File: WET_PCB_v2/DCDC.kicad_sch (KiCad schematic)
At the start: 8 parts, among them Q5 Q_NMOS_GDS, Q6 Q_NMOS_GDS

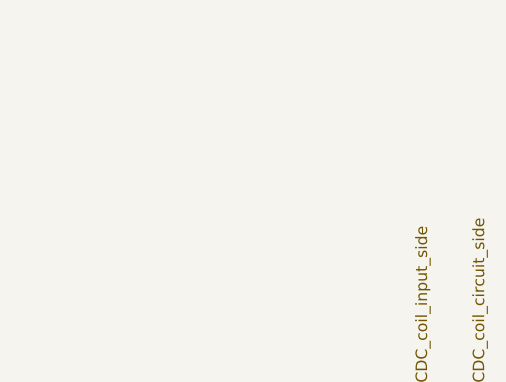
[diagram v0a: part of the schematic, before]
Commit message: finished and added some drawings
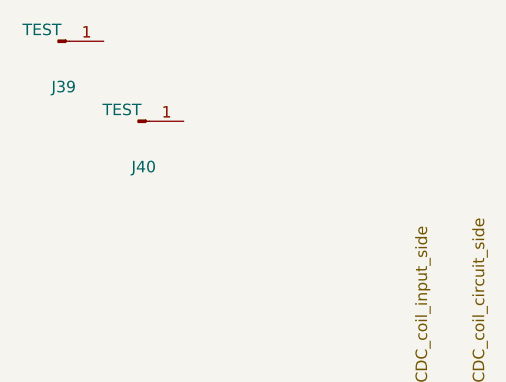
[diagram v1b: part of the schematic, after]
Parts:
- added J39, J40: TEST, Connector_PinSocket_2.54mm:PinSocket_1x01_P2.54mm_Vertical, symbol Connector:Conn_01x01_Pin
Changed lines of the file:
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@@
+	)
+	(symbol
+		(lib_id "Connector:Conn_01x01_Pin")
+		(at 12.926 11.1816 0)
+		(unit 1)
+		(body_style 1)
+		(exclude_from_sim no)
+		(in_bom yes)
+		(on_board yes)
+		(in_pos_files yes)
+		(dnp no)
+		(property "Reference" "J40"
+			(at 13.561 16.2616 0)
+			(show_name no)
+			(do_not_autoplace no)
+			(effects
+				(font
+					(size 1.27 1.27)
+				)
+			)
+		)
+		(property "Value" "TEST"
+			(at 11.148 9.9116 0)
+			(show_name no)
+			(do_not_autoplace no)
+			(effects
+				(font
+					(size 1.27 1.27)
+				)
+			)
+		)
+		(property "Footprint" "Connector_PinSocket_2.54mm:PinSocket_1x01_P2.54mm_Vertical"
+			(at 12.926 11.1816 0)
+			(hide yes)
+			(show_name no)
+			(do_not_autoplace no)
+			(effects
+				(font
+					(size 1.27 1.27)
+				)
+			)
+		)
+		(property "Datasheet" ""
+			(at 12.926 11.1816 0)
+			(hide yes)
+			(show_name no)
+			(do_not_autoplace no)
+			(effects
+				(font
+					(size 1.27 1.27)
+				)
+			)
+		)
+		(property "Description" "Generic connector, single row, 01x01, script generated"
+			(at 12.926 11.1816 0)
+			(hide yes)
+			(show_name no)
+			(do_not_autoplace no)
+			(effects
+				(font
+					(size 1.27 1.27)
+				)
+			)
+		)
+		(pin "1"
+		)
+		(instances
+			(project "WET_PCB_v2"
+				(path "/13451c35-1666-47d9-9525-8d8125ba1cf3/04007180-46fe-4cf0-9e6f-a7d321798318"
+					(reference "J40")
+					(unit 1)
+				)
+			)
+		)
+	)
+	(symbol
+		(lib_id "Connector:Conn_01x01_Pin")
+		(at 4.036 2.2916 0)
+		(unit 1)
+		(body_style 1)
+		(exclude_from_sim no)
+		(in_bom yes)
+		(on_board yes)
+		(in_pos_files yes)
+		(dnp no)
+		(property "Reference" "J39"
+			(at 4.671 7.3716 0)
+			(show_name no)
+			(do_not_autoplace no)
+			(effects
+				(font
+					(size 1.27 1.27)
+				)
+			)
+		)
+		(property "Value" "TEST"
+			(at 2.258 1.0216 0)
+			(show_name no)
+			(do_not_autoplace no)
+			(effects
+				(font
+					(size 1.27 1.27)
+				)
+			)
+		)
+		(property "Footprint" "Connector_PinSocket_2.54mm:PinSocket_1x01_P2.54mm_Vertical"
+			(at 4.036 2.2916 0)
+			(hide yes)
+			(show_name no)
+			(do_not_autoplace no)
+			(effects
+				(font
+					(size 1.27 1.27)
+				)
+			)
+		)
+		(property "Datasheet" ""
+			(at 4.036 2.2916 0)
+			(hide yes)
+			(show_name no)
+			(do_not_autoplace no)
+			(effects
+				(font
+					(size 1.27 1.27)
+				)
+			)
+		)
+		(property "Description" "Generic connector, single row, 01x01, script generated"
+			(at 4.036 2.2916 0)
+			(hide yes)
+			(show_name no)
+			(do_not_autoplace no)
+			(effects
+				(font
+					(size 1.27 1.27)
+				)
+			)
+		)
+		(pin "1"
+		)
+		(instances
+			(project "WET_PCB_v2"
+				(path "/13451c35-1666-47d9-9525-8d8125ba1cf3/04007180-46fe-4cf0-9e6f-a7d321798318"
+					(reference "J39")
+					(unit 1)
+				)
+			)
+		)
 	)
 	(symbol

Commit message: cleaned up schematics, added power LED
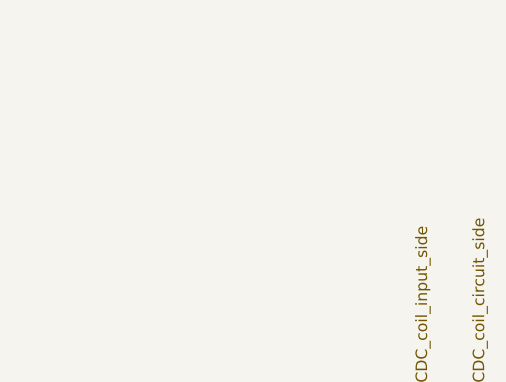
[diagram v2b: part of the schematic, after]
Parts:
- removed J39, J40: TEST, Connector_PinSocket_2.54mm:PinSocket_1x01_P2.54mm_Vertical, symbol Connector:Conn_01x01_Pin
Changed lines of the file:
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@@
-	)
-	(symbol
-		(lib_id "Connector:Conn_01x01_Pin")
-		(at 12.926 11.1816 0)
-		(unit 1)
-		(body_style 1)
-		(exclude_from_sim no)
-		(in_bom yes)
-		(on_board yes)
-		(in_pos_files yes)
-		(dnp no)
-		(property "Reference" "J40"
-			(at 13.561 16.2616 0)
-			(show_name no)
-			(do_not_autoplace no)
-			(effects
-				(font
-					(size 1.27 1.27)
-				)
-			)
-		)
-		(property "Value" "TEST"
-			(at 11.148 9.9116 0)
-			(show_name no)
-			(do_not_autoplace no)
-			(effects
-				(font
-					(size 1.27 1.27)
-				)
-			)
-		)
-		(property "Footprint" "Connector_PinSocket_2.54mm:PinSocket_1x01_P2.54mm_Vertical"
-			(at 12.926 11.1816 0)
-			(hide yes)
-			(show_name no)
-			(do_not_autoplace no)
-			(effects
-				(font
-					(size 1.27 1.27)
-				)
-			)
-		)
-		(property "Datasheet" ""
-			(at 12.926 11.1816 0)
-			(hide yes)
-			(show_name no)
-			(do_not_autoplace no)
-			(effects
-				(font
-					(size 1.27 1.27)
-				)
-			)
-		)
-		(property "Description" "Generic connector, single row, 01x01, script generated"
-			(at 12.926 11.1816 0)
-			(hide yes)
-			(show_name no)
-			(do_not_autoplace no)
-			(effects
-				(font
-					(size 1.27 1.27)
-				)
-			)
-		)
-		(pin "1"
-		)
-		(instances
-			(project "WET_PCB_v2"
-				(path "/13451c35-1666-47d9-9525-8d8125ba1cf3/04007180-46fe-4cf0-9e6f-a7d321798318"
-					(reference "J40")
-					(unit 1)
-				)
-			)
-		)
-	)
-	(symbol
-		(lib_id "Connector:Conn_01x01_Pin")
-		(at 4.036 2.2916 0)
-		(unit 1)
-		(body_style 1)
-		(exclude_from_sim no)
-		(in_bom yes)
-		(on_board yes)
-		(in_pos_files yes)
-		(dnp no)
-		(property "Reference" "J39"
-			(at 4.671 7.3716 0)
-			(show_name no)
-			(do_not_autoplace no)
-			(effects
-				(font
-					(size 1.27 1.27)
-				)
-			)
-		)
-		(property "Value" "TEST"
-			(at 2.258 1.0216 0)
-			(show_name no)
-			(do_not_autoplace no)
-			(effects
-				(font
-					(size 1.27 1.27)
-				)
-			)
-		)
-		(property "Footprint" "Connector_PinSocket_2.54mm:PinSocket_1x01_P2.54mm_Vertical"
-			(at 4.036 2.2916 0)
-			(hide yes)
-			(show_name no)
-			(do_not_autoplace no)
-			(effects
-				(font
-					(size 1.27 1.27)
-				)
-			)
-		)
-		(property "Datasheet" ""
-			(at 4.036 2.2916 0)
-			(hide yes)
-			(show_name no)
-			(do_not_autoplace no)
-			(effects
-				(font
-					(size 1.27 1.27)
-				)
-			)
-		)
-		(property "Description" "Generic connector, single row, 01x01, script generated"
-			(at 4.036 2.2916 0)
-			(hide yes)
-			(show_name no)
-			(do_not_autoplace no)
-			(effects
-				(font
-					(size 1.27 1.27)
-				)
-			)
-		)
-		(pin "1"
-		)
-		(instances
-			(project "WET_PCB_v2"
-				(path "/13451c35-1666-47d9-9525-8d8125ba1cf3/04007180-46fe-4cf0-9e6f-a7d321798318"
-					(reference "J39")
-					(unit 1)
-				)
-			)
-		)
 	)
 	(symbol
